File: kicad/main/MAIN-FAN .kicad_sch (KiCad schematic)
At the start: 9 parts, among them Q1 AO4407A, Q9 IRLML6344TRPBF

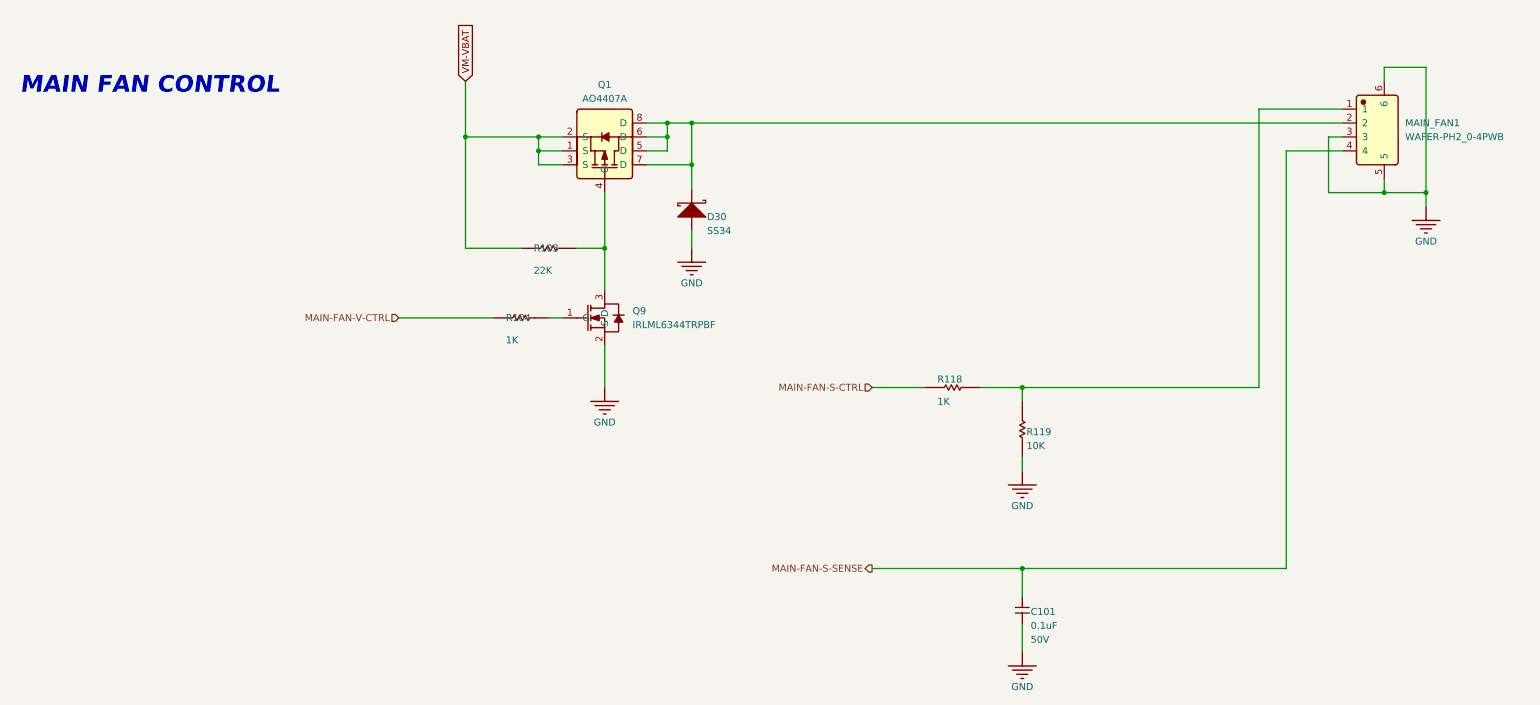
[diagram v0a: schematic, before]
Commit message: Schematic fixes, 1st round of review
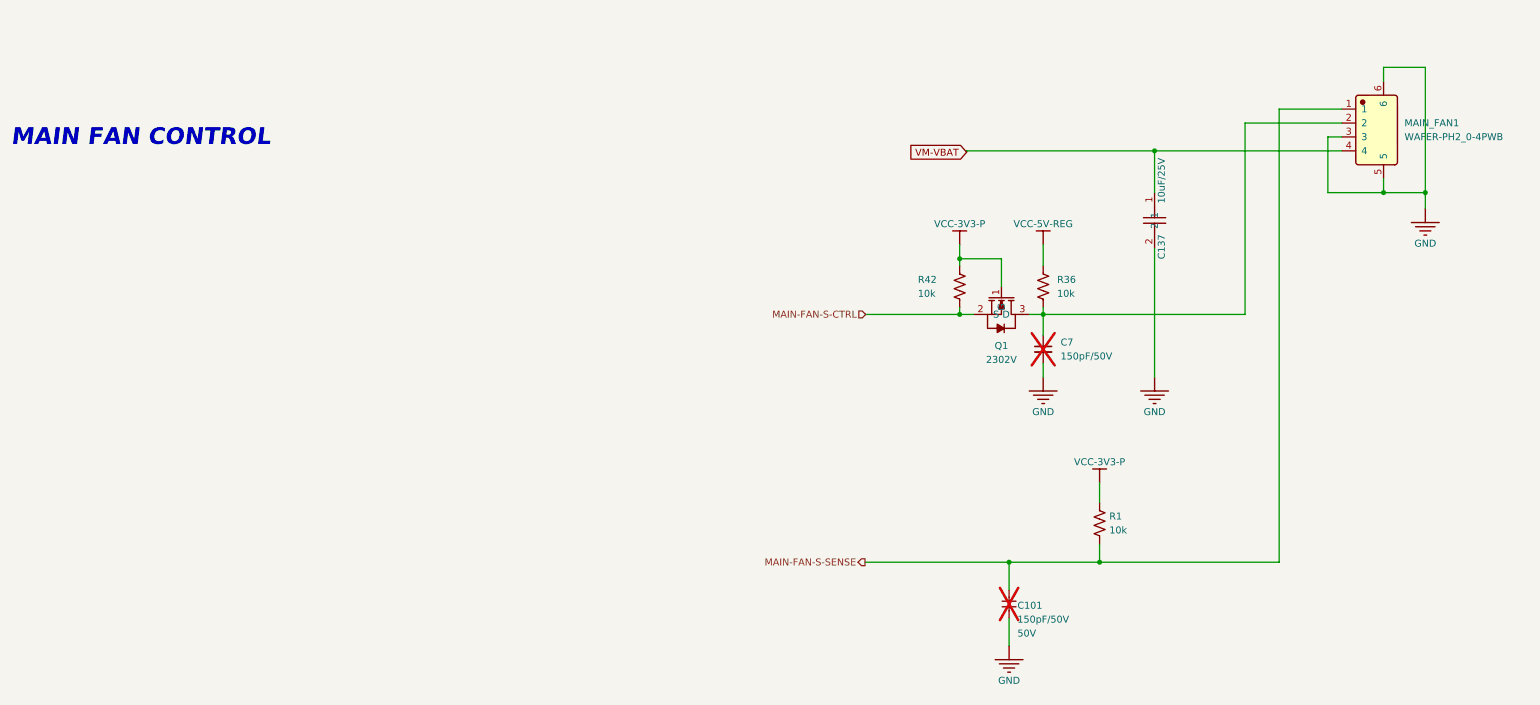
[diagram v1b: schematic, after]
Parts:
- removed D30: SS34, oomwoo_altium:SMA, symbol DesignLibrary:MAIN-BRUSH MOTOR_1_DIODE-2_DesignLibrary.SchLib
- removed Q1: AO4407A, JLCImport:AO4407A, symbol JLCImport:AO4407A
- removed Q9: IRLML6344TRPBF, JLCImport:IRLML6344TRPBF, symbol JLCImport:IRLML6344TRPBF
- removed R103: 22K, Resistor_SMD:R_0603_1608Metric, symbol DesignLibrary:MAIN-FAN_0_Resistor-1_DesignLibrary.SchLib
- removed R104: 1K, Resistor_SMD:R_0603_1608Metric, symbol DesignLibrary:MAIN-FAN_0_Resistor-1_DesignLibrary.SchLib
- removed R118: 1K, Resistor_SMD:R_0603_1608Metric, symbol DesignLibrary:MAIN-FAN_2_Resistor-1_DesignLibrary.SchLib
- removed R119: 10K, Resistor_SMD:R_0603_1608Metric, symbol DesignLibrary:MAIN-FAN_1_Resistor-1_DesignLibrary.SchLib
- added C137: 10uF/25V, Capacitor_SMD:C_0603_1608Metric, symbol JLCImport:CL21A106KBYQNNE
- added C7: 150pF/50V, Capacitor_SMD:C_0603_1608Metric, symbol Device:C_Small
- added Q1: 2302V, JLCImport:2302V, symbol JLCImport:2302V
- added R1, R36, R42: 10k, Resistor_SMD:R_0603_1608Metric, symbol Device:R_US
- C101: value 0.1uF -> 150pF/50V; MANUFACTURER * -> (none); Manufacturer (none) -> *; now not fitted
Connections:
- net GND: now also C137.2, C7.2
- net MAIN-FAN-S-CTRL: now also Q1.2 (S), R42.2
- net MAIN-FAN-S-SENSE: now also MAIN_FAN1.1, R1.2; no longer MAIN_FAN1.4
- net VM-VBAT: now also MAIN_FAN1.4, C137.1
- net at MAIN_FAN1.2: now also C7.1, Q1.3 (D), R36.2
- new net VCC-3V3-P: Q1.1 (G), R1.1, R42.1
- new net VCC-5V-REG: R36.1
